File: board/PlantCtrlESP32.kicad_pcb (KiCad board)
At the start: 2 copper layers, 99.1 x 99.1 mm, 163 parts, among them J1 Conn_01x03_Female, Q1 N-channel 30V 5A, Q10 N-channel 30V 5A, Q11 N-channel 30V 5A, Q2 N-channel 30V 5A, Q3 N-channel 30V 5A, Q4 N-channel 30V 5A, Q5 N-channel 30V 5A, Q6 N-channel 30V 5A, Q7 N-channel 30V 5A, Q8 N-channel 30V 5A, Q9 N-channel 30V 5A, U1 DS18B20, U2 ds2438az+, U3 LP38690DT-3.3, U4 SX1308, U5 ESP32-WROOM-32D, U6 CN61CN33

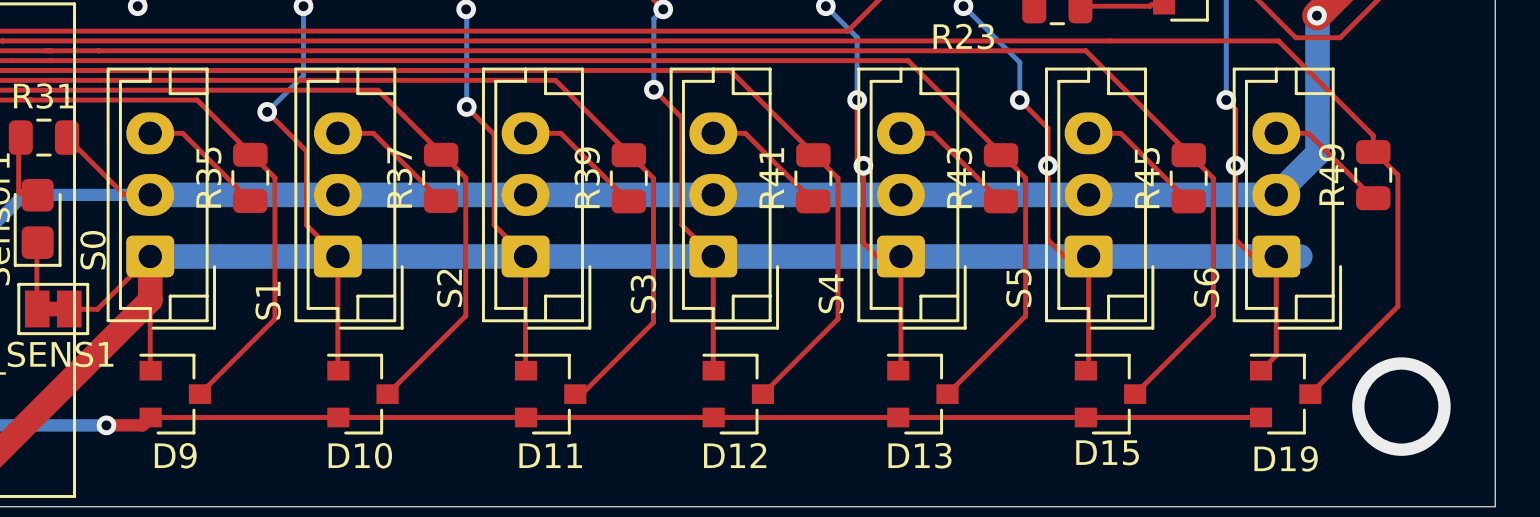
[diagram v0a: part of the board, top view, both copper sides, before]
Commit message: add high impendance pulldown to analog in
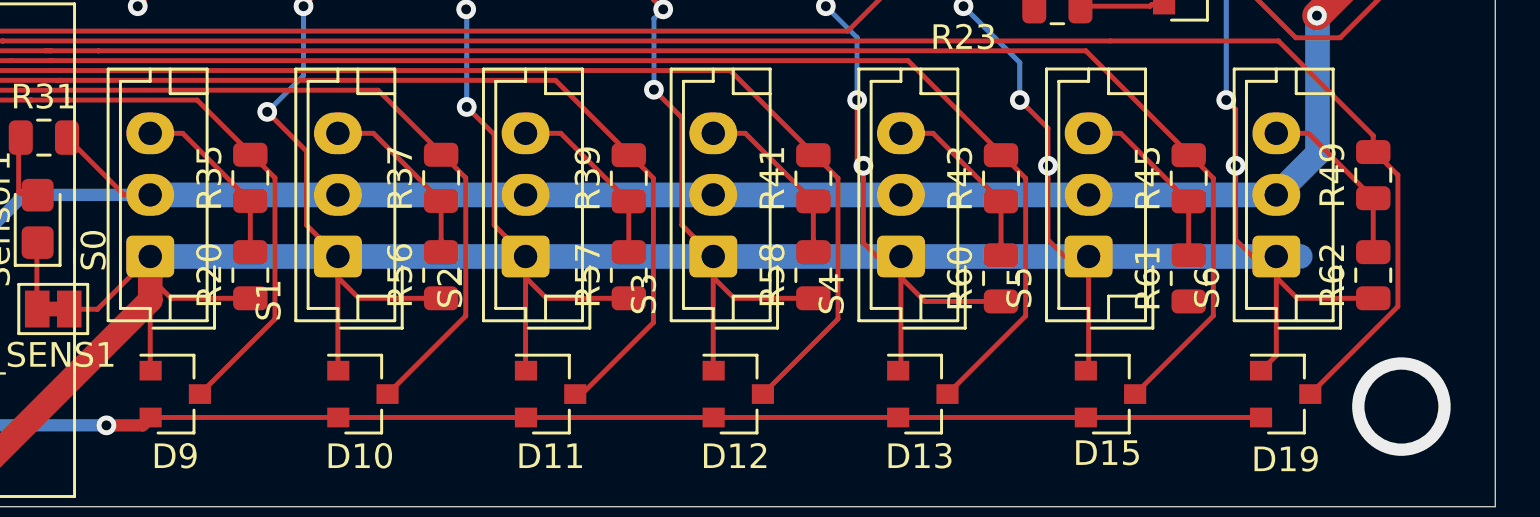
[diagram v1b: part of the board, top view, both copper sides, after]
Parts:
- added R20: 100k, Resistor_SMD:R_0805_2012Metric, F.Cu at (218.7, 130.3)
- added R56: 100k, Resistor_SMD:R_0805_2012Metric, F.Cu at (226.4, 130.3)
- added R57: 100k, Resistor_SMD:R_0805_2012Metric, F.Cu at (234.1, 130.3)
- added R58: 100k, Resistor_SMD:R_0805_2012Metric, F.Cu at (241.6, 130.3)
- added R60: 100k, Resistor_SMD:R_0805_2012Metric, F.Cu at (249.2, 130.4)
- added R61: 100k, Resistor_SMD:R_0805_2012Metric, F.Cu at (256.8, 130.4)
- added R62: 100k, Resistor_SMD:R_0805_2012Metric, F.Cu at (264.3, 130.3)
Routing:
- net GND: track 1322.8 -> 1354.6 mm
- net Net-(R45-Pad1): track 5.67 -> 7.86 mm
- net Net-(R43-Pad1): track 5.67 -> 7.86 mm
- net Net-(R49-Pad1): track 5.56 -> 7.75 mm
- net Net-(R37-Pad1): track 5.77 -> 7.84 mm
- net Net-(R20-Pad2): track 5.88 -> 7.96 mm
- net Net-(R41-Pad1): track 5.67 -> 7.73 mm
- net Net-(R39-Pad1): track 5.79 -> 7.86 mm
